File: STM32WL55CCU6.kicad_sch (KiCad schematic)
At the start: 31 parts, among them J6 BOOT0_Jumper, SW3 Switch_NX3L1T3157GM,115, U4 STM32WL55CCU6

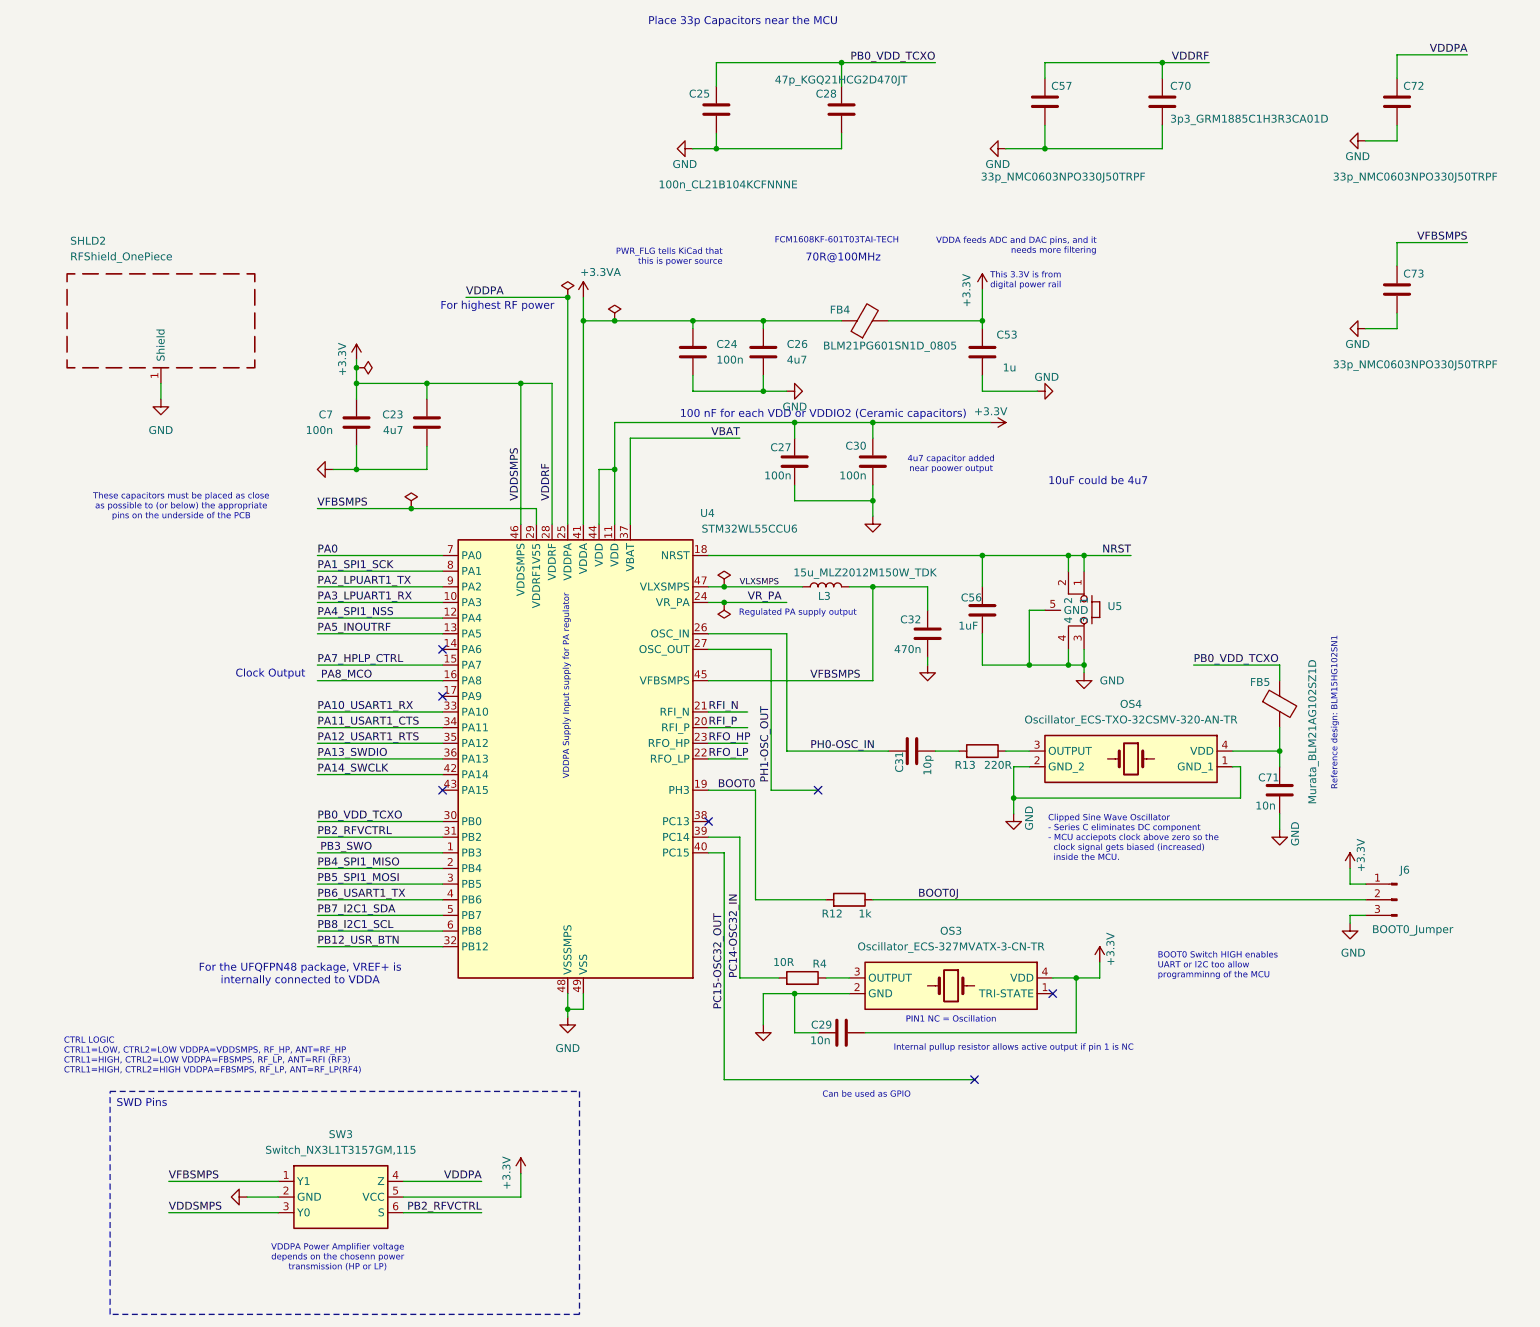
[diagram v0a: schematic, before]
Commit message: Update
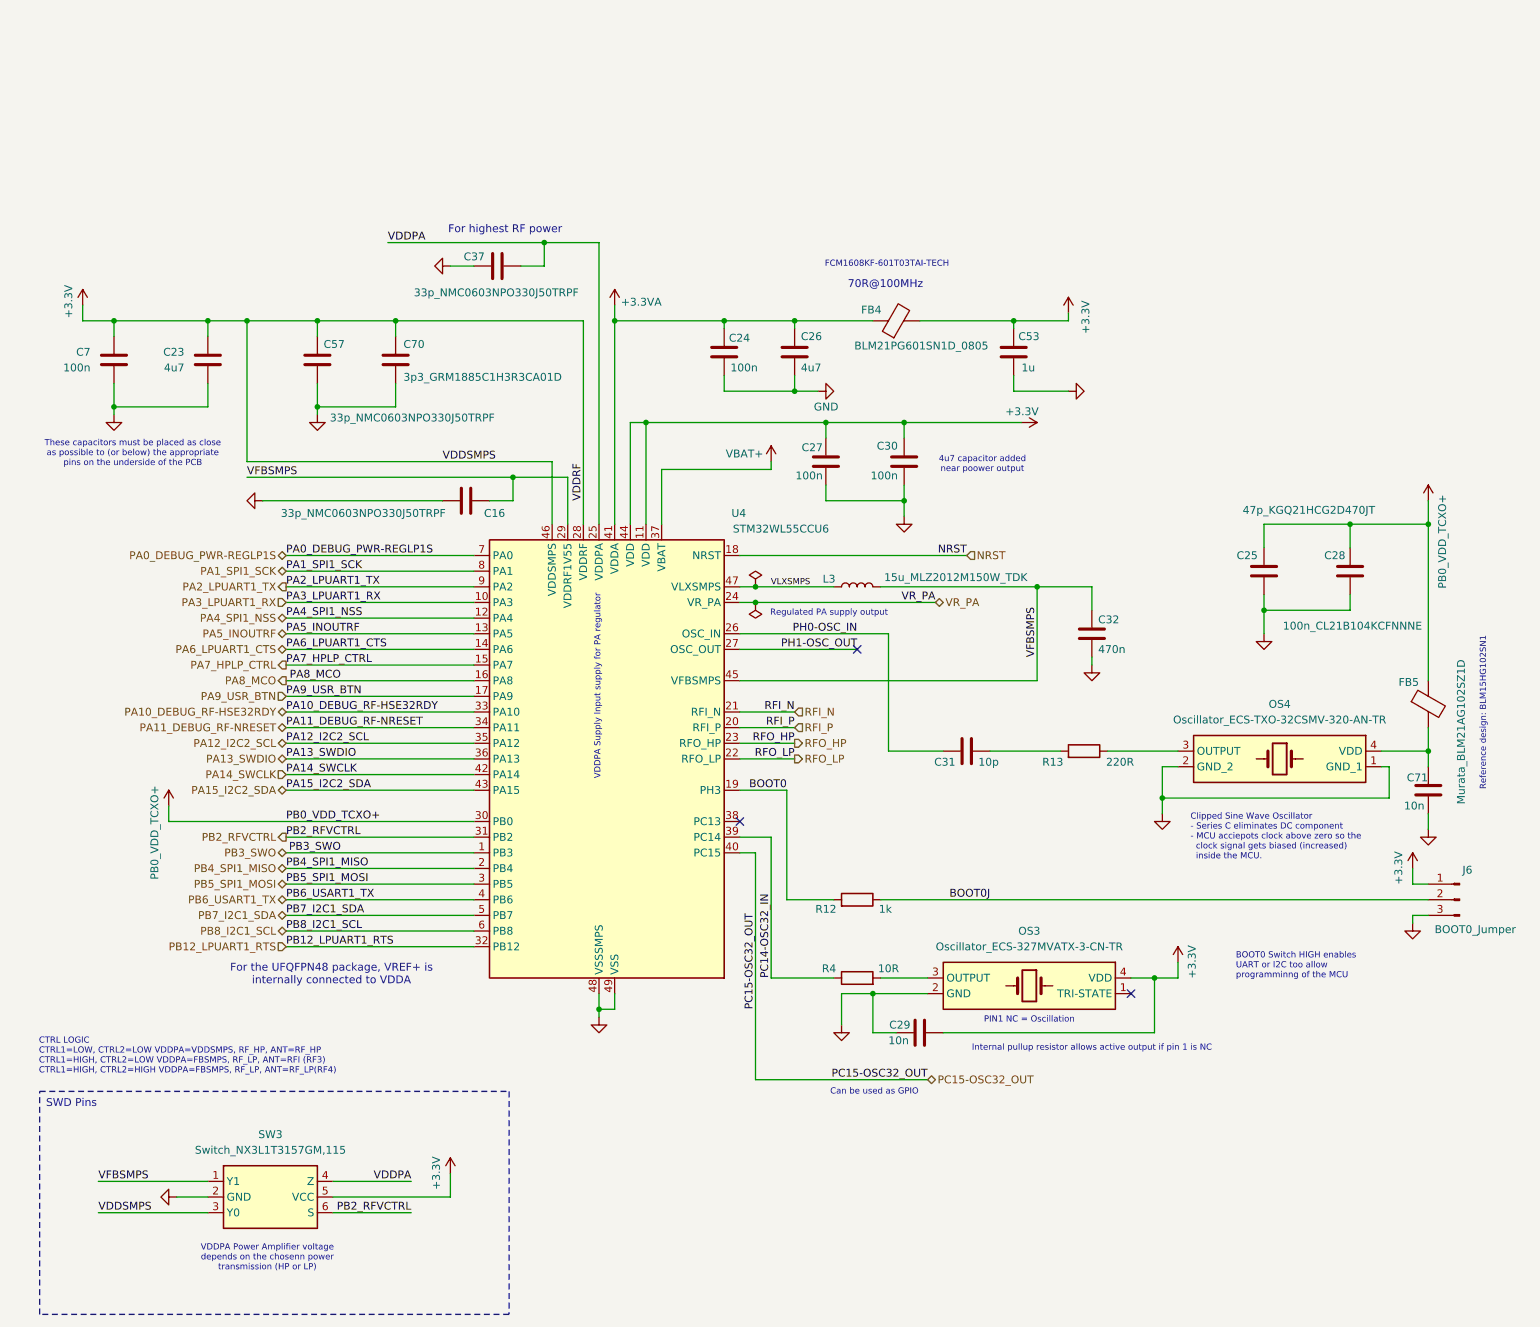
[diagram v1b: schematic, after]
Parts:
- removed C56: 1uF, Capacitor_SMD:C_0805_2012Metric, symbol Device:C
- removed C72, C73: 33p_NMC0603NPO330J50TRPF, Capacitor_SMD:C_0603_1608Metric, symbol Device:C
- removed SHLD2: RFShield_OnePiece, Personal_Project:RF_Shield_MS631-10F, symbol Device:RFShield_OnePiece
- removed U5: ~, Personal_Project:Button_KMR231GLFS, symbol Personal_Projects:Button_KMR231GLFS
- added C16, C37: 33p_NMC0603NPO330J50TRPF, Capacitor_SMD:C_0603_1608Metric, symbol Device:C
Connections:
- net GND: now also C16.1, C37.1
- net PC14-OSC32_IN: now also R4.1; no longer R4.2
- net VDDPA: now also C37.2
- net VFBSMPS: now also C16.2
- net at OS3.3 (OUTPUT): now also R4.2; no longer R4.1
- net PA6_LPUART1_CTS: now reaches U4.14 (PA6)
- net PA9_USR_BTN: now reaches U4.17 (PA9)
- net PA15_I2C2_SDA: now reaches U4.43 (PA15)
- net PA0 renamed PA0_DEBUG_PWR-REGLP1S
- net PA10_USART1_RX renamed PA10_DEBUG_RF-HSE32RDY
- net PA11_USART1_CTS renamed PA11_DEBUG_RF-NRESET
- net PA12_USART1_RTS renamed PA12_I2C2_SCL
- net PB0_VDD_TCXO renamed PB0_VDD_TCXO+
- net PB12_USR_BTN renamed PB12_LPUART1_RTS
- net VBAT renamed VBAT+
- no-connect marks 7 -> 3
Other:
- note removed: "100 nF for each VDD or VDDIO2 (Ceramic capacitors)"
- note removed: "10uF could be 4u7"
- note removed: "Clock Output"
- note removed: "PWR_FLG tells KiCad that this is power source"
- note removed: "Place 33p Capacitors near the MCU"
- note removed: "This 3.3V is from digital power rail"
- note removed: "VDDA feeds ADC and DAC pins, and it needs more filtering"
- title: (none) -> LORA_STM32WL55CCU6_Board
- moved on the sheet: C23, C24, C25, C26, C27, C28, C29, C30, C31, C32, C53, C57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
